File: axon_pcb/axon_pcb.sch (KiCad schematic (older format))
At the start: 106 parts, among them J1 USB_C_Receptacle, J2 AVR_ISP Header, K1 KEYSW, K10 KEYSW, K11 KEYSW, K12 KEYSW, K13 KEYSW, K14 KEYSW, K15 KEYSW, K16 KEYSW, K17 KEYSW, K18 KEYSW, K19 KEYSW, K2 KEYSW, K20 KEYSW, K21 KEYSW, K22 KEYSW, K23 KEYSW, K24 KEYSW, K25 KEYSW, K26 KEYSW, K27 KEYSW, K28 KEYSW, K29 KEYSW, K3 KEYSW, K30 KEYSW, K31 KEYSW, K32 KEYSW, K33 KEYSW, K34 KEYSW, K35 KEYSW, K36 KEYSW, K37 KEYSW, K38 KEYSW, K39 KEYSW, K4 KEYSW, K40 KEYSW, K41 KEYSW, K42 KEYSW, K43 KEYSW, K44 KEYSW, K45 KEYSW, K46 KEYSW, K5 KEYSW, K6 KEYSW, K7 KEYSW, K8 KEYSW, K9 KEYSW, SW1 RESET, SW2 BOOT, U1 ATmega328P-PU, X1 16MHz

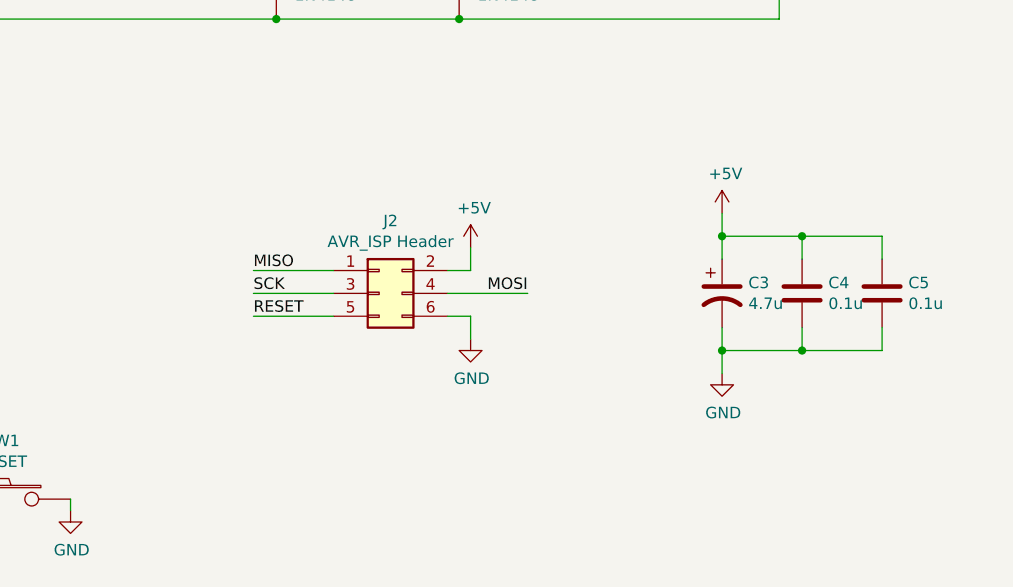
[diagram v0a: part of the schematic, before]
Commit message: add power LED
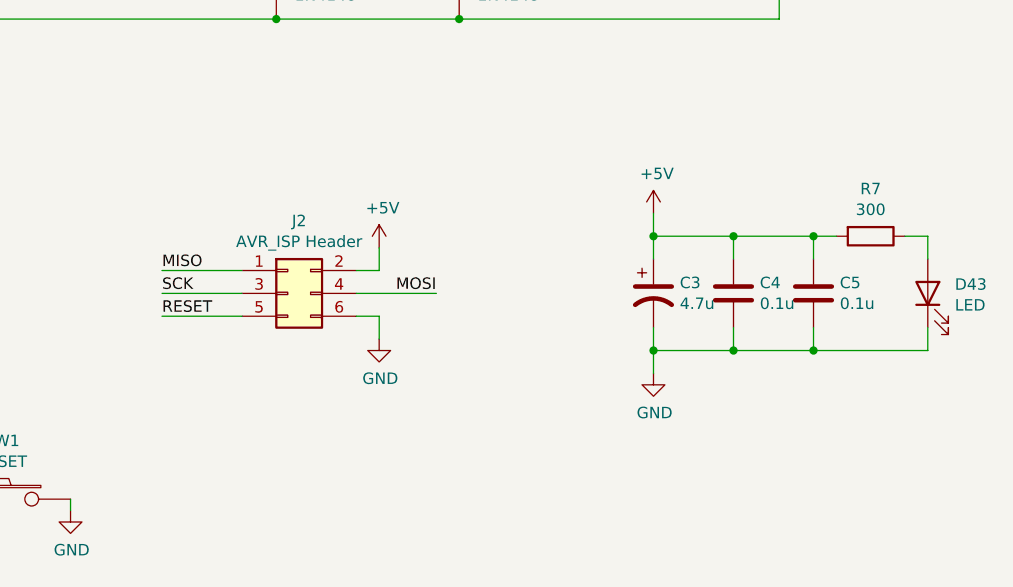
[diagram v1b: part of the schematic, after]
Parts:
- added D43: LED, LED_THT:LED_D5.0mm, symbol Device:LED
- added R7: 300, Resistor_THT:R_Axial_DIN0204_L3.6mm_D1.6mm_P5.08mm_Horizontal, symbol Device:R
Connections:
- net +5V: now also R7.2
- net GND: now also D43.1 (K)
- new net: D43.2 (A), R7.1
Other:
- moved on the sheet: C3, C4, C5, J2
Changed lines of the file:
@@
 $EndComp
 Wire Wire Line
-	9650 5200 10000 5200
-Wire Wire Line
-	9650 5800 9650 5700
-Wire Wire Line
-	9650 5700 10000 5700
+	9350 5200 9700 5200
+Wire Wire Line
+	9350 5800 9350 5700
+Wire Wire Line
+	9350 5700 9700 5700
 $Comp
 L power:GND #PWR0104
 U 1 1 605AEB44
-P 9650 5800
-F 0 "#PWR0104" H 9650 5550 50  0001 C CNN
-F 1 "GND" H 9655 5627 50  0000 C CNN
-F 2 "" H 9650 5800 50  0001 C CNN
-F 3 "" H 9650 5800 50  0001 C CNN
-	1    9650 5800
+P 9350 5800
+F 0 "#PWR0104" H 9350 5550 50  0001 C CNN
+F 1 "GND" H 9355 5627 50  0000 C CNN
+F 2 "" H 9350 5800 50  0001 C CNN
+F 3 "" H 9350 5800 50  0001 C CNN
+	1    9350 5800
 	1    0    0    -1
 $EndComp
@@
 L Device:C C5
 U 1 1 605B014B
-P 10350 5450
-F 0 "C5" H 10465 5496 50  0000 L CNN
-F 1 "0.1u" H 10465 5405 50  0000 L CNN
-F 2 "Capacitor_THT:C_Disc_D4.3mm_W1.9mm_P5.00mm" H 10388 5300 50  0001 C CNN
-F 3 "~" H 10350 5450 50  0001 C CNN
-	1    10350 5450
+P 10050 5450
+F 0 "C5" H 10165 5496 50  0000 L CNN
+F 1 "0.1u" H 10165 5405 50  0000 L CNN
+F 2 "Capacitor_THT:C_Disc_D4.3mm_W1.9mm_P5.00mm" H 10088 5300 50  0001 C CNN
+F 3 "~" H 10050 5450 50  0001 C CNN
+	1    10050 5450
 	1    0    0    -1
 $EndComp
@@
 L Device:C C4
 U 1 1 605B0B1A
-P 10000 5450
-F 0 "C4" H 10115 5496 50  0000 L CNN
-F 1 "0.1u" H 10115 5405 50  0000 L CNN
-F 2 "Capacitor_THT:C_Disc_D4.3mm_W1.9mm_P5.00mm" H 10038 5300 50  0001 C CNN
-F 3 "~" H 10000 5450 50  0001 C CNN
-	1    10000 5450
-	1    0    0    -1
-$EndComp
-Wire Wire Line
-	9650 5600 9650 5700
-Connection ~ 9650 5700
-Wire Wire Line
-	10000 5600 10000 5700
-Wire Wire Line
-	10000 5300 10000 5200
-Wire Wire Line
-	9650 5300 9650 5200
+P 9700 5450
+F 0 "C4" H 9815 5496 50  0000 L CNN
+F 1 "0.1u" H 9815 5405 50  0000 L CNN
+F 2 "Capacitor_THT:C_Disc_D4.3mm_W1.9mm_P5.00mm" H 9738 5300 50  0001 C CNN
+F 3 "~" H 9700 5450 50  0001 C CNN
+	1    9700 5450
+	1    0    0    -1
+$EndComp
+Wire Wire Line
+	9350 5600 9350 5700
+Connection ~ 9350 5700
+Wire Wire Line
+	9700 5600 9700 5700
+Wire Wire Line
+	9700 5300 9700 5200
+Wire Wire Line
+	9350 5300 9350 5200
 $Comp
 L power:+5V #PWR0105
 U 1 1 605C0C6E
-P 9650 5100
-F 0 "#PWR0105" H 9650 4950 50  0001 C CNN
-F 1 "+5V" H 9665 5273 50  0000 C CNN
-F 2 "" H 9650 5100 50  0001 C CNN
-F 3 "" H 9650 5100 50  0001 C CNN
-	1    9650 5100
-	1    0    0    -1
-$EndComp
-Wire Wire Line
-	9650 5100 9650 5200
-Connection ~ 9650 5200
+P 9350 5100
+F 0 "#PWR0105" H 9350 4950 50  0001 C CNN
+F 1 "+5V" H 9365 5273 50  0000 C CNN
+F 2 "" H 9350 5100 50  0001 C CNN
+F 3 "" H 9350 5100 50  0001 C CNN
+	1    9350 5100
+	1    0    0    -1
+$EndComp
+Wire Wire Line
+	9350 5100 9350 5200
+Connection ~ 9350 5200
 $Comp
 L keyboard-parts:SW_PUSH SW1
@@
 L Device:CP1 C3
 U 1 1 60636CDE
-P 9650 5450
-F 0 "C3" H 9765 5496 50  0000 L CNN
-F 1 "4.7u" H 9765 5405 50  0000 L CNN
-F 2 "Capacitor_THT:CP_Radial_D4.0mm_P1.50mm" H 9650 5450 50  0001 C CNN
-F 3 "~" H 9650 5450 50  0001 C CNN
-	1    9650 5450
-	1    0    0    -1
-$EndComp
-Wire Wire Line
-	10000 5200 10350 5200
-Wire Wire Line
-	10350 5200 10350 5300
-Connection ~ 10000 5200
-Wire Wire Line
-	10350 5600 10350 5700
-Wire Wire Line
-	10350 5700 10000 5700
-Connection ~ 10000 5700
+P 9350 5450
+F 0 "C3" H 9465 5496 50  0000 L CNN
+F 1 "4.7u" H 9465 5405 50  0000 L CNN
+F 2 "Capacitor_THT:CP_Radial_D4.0mm_P1.50mm" H 9350 5450 50  0001 C CNN
+F 3 "~" H 9350 5450 50  0001 C CNN
+	1    9350 5450
+	1    0    0    -1
+$EndComp
+Wire Wire Line
+	9700 5200 10050 5200
+Wire Wire Line
+	10050 5200 10050 5300
+Connection ~ 9700 5200
+Wire Wire Line
+	10050 5600 10050 5700
+Wire Wire Line
+	10050 5700 9700 5700
+Connection ~ 9700 5700
 $Comp
 L Connector_Generic:Conn_02x03_Odd_Even J2
 U 1 1 606EAAB0
-P 8150 5450
-F 0 "J2" H 8200 5767 50  0000 C CNN
-F 1 "AVR_ISP Header" H 8200 5676 50  0000 C CNN
-F 2 "personal:PinHeader_2x03_P2.54mm_Vertical" H 8150 5450 50  0001 C CNN
-F 3 "~" H 8150 5450 50  0001 C CNN
-	1    8150 5450
-	1    0    0    -1
-$EndComp
-Wire Wire Line
-	7950 5550 7600 5550
-Text Label 7600 5550 0    50   ~ 0
+P 7750 5450
+F 0 "J2" H 7800 5767 50  0000 C CNN
+F 1 "AVR_ISP Header" H 7800 5676 50  0000 C CNN
+F 2 "personal:PinHeader_2x03_P2.54mm_Vertical" H 7750 5450 50  0001 C CNN
+F 3 "~" H 7750 5450 50  0001 C CNN
+	1    7750 5450
+	1    0    0    -1
+$EndComp
+Wire Wire Line
+	7550 5550 7200 5550
+Text Label 7200 5550 0    50   ~ 0
 RESET
 Text Label 5150 6350 2    50   ~ 0
@@
 	4800 5150 5150 5150
 Wire Wire Line
-	8450 5550 8550 5550
-Wire Wire Line
-	8550 5550 8550 5650
+	8050 5550 8150 5550
+Wire Wire Line
+	8150 5550 8150 5650
 $Comp
 L power:GND #PWR0108
 U 1 1 60729A0A
-P 8550 5650
-F 0 "#PWR0108" H 8550 5400 50  0001 C CNN
-F 1 "GND" H 8555 5477 50  0000 C CNN
-F 2 "" H 8550 5650 50  0001 C CNN
-F 3 "" H 8550 5650 50  0001 C CNN
-	1    8550 5650
-	1    0    0    -1
-$EndComp
-Wire Wire Line
-	8450 5350 8550 5350
-Wire Wire Line
-	8550 5350 8550 5250
+P 8150 5650
+F 0 "#PWR0108" H 8150 5400 50  0001 C CNN
+F 1 "GND" H 8155 5477 50  0000 C CNN
+F 2 "" H 8150 5650 50  0001 C CNN
+F 3 "" H 8150 5650 50  0001 C CNN
+	1    8150 5650
+	1    0    0    -1
+$EndComp
+Wire Wire Line
+	8050 5350 8150 5350
+Wire Wire Line
+	8150 5350 8150 5250
 Wire Wire Line
 	1700 5350 1700 5400
@@
 	1700 5600 1700 5650
 Wire Wire Line
-	8450 5450 8800 5450
-Wire Wire Line
-	7950 5450 7600 5450
-Wire Wire Line
-	7950 5350 7600 5350
-Text Label 7600 5450 0    50   ~ 0
+	8050 5450 8400 5450
+Wire Wire Line
+	7550 5450 7200 5450
+Wire Wire Line
+	7550 5350 7200 5350
+Text Label 7200 5450 0    50   ~ 0
 SCK
-Text Label 7600 5350 0    50   ~ 0
+Text Label 7200 5350 0    50   ~ 0
 MISO
-Text Label 8800 5450 2    50   ~ 0
+Text Label 8400 5450 2    50   ~ 0
 MOSI
 Text Label 5150 5150 2    50   ~ 0
@@
 L power:+5V #PWR0109
 U 1 1 61A2F4BB
-P 8550 5250
-F 0 "#PWR0109" H 8550 5100 50  0001 C CNN
-F 1 "+5V" H 8565 5423 50  0000 C CNN
-F 2 "" H 8550 5250 50  0001 C CNN
-F 3 "" H 8550 5250 50  0001 C CNN
-	1    8550 5250
+P 8150 5250
+F 0 "#PWR0109" H 8150 5100 50  0001 C CNN
+F 1 "+5V" H 8165 5423 50  0000 C CNN
+F 2 "" H 8150 5250 50  0001 C CNN
+F 3 "" H 8150 5250 50  0001 C CNN
+	1    8150 5250
 	1    0    0    -1
 $EndComp
@@
 Text Notes 9150 3450 0    50   ~ 0
 1u
+$Comp
+L Device:R R7
+U 1 1 61A4F81C
+P 10300 5200
+F 0 "R7" V 10093 5200 50  0000 C CNN
+F 1 "300" V 10184 5200 50  0000 C CNN
+F 2 "Resistor_THT:R_Axial_DIN0204_L3.6mm_D1.6mm_P5.08mm_Horizontal" V 10230 5200 50  0001 C CNN
+F 3 "~" H 10300 5200 50  0001 C CNN
+	1    10300 5200
+	0    1    1    0
+$EndComp
+Wire Wire Line
+	10050 5200 10150 5200
+Connection ~ 10050 5200
+$Comp
+L Device:LED D43
+U 1 1 61A5C4D6
+P 10550 5450
+F 0 "D43" V 10589 5332 50  0000 R CNN
+F 1 "LED" V 10498 5332 50  0000 R CNN
+F 2 "LED_THT:LED_D5.0mm" H 10550 5450 50  0001 C CNN
+F 3 "~" H 10550 5450 50  0001 C CNN
+	1    10550 5450
+	0    -1   -1   0
+$EndComp
+Wire Wire Line
+	10450 5200 10550 5200
+Wire Wire Line
+	10550 5200 10550 5300
+Wire Wire Line
+	10550 5600 10550 5700
+Wire Wire Line
+	10550 5700 10050 5700
+Connection ~ 10050 5700
 $EndSCHEMATC
